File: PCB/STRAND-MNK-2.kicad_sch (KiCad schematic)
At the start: 4 parts

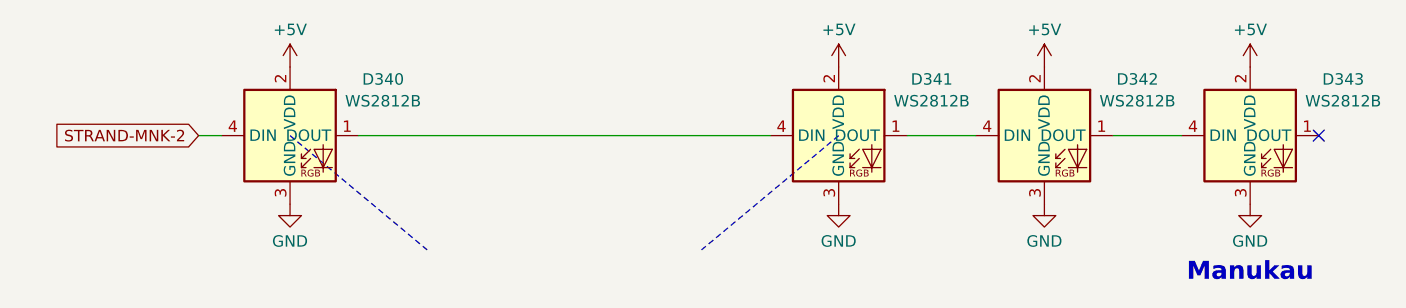
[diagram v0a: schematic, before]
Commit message: Final tweaks for V1.0.0
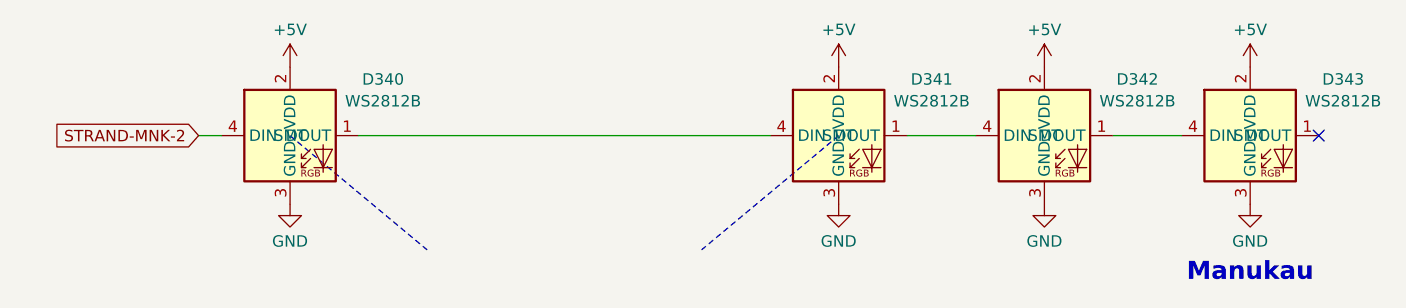
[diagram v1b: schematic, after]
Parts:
- D340, D341, D342, D343: Manufacturer (none) -> XINGLIGHT; Part (none) -> XL-1615RGBC-WS2812B; Process (none) -> SMT
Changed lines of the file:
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@@
+			)
+		)
+		(property "Part" "XL-1615RGBC-WS2812B"
+			(at 124.46 27.94 0)
+			(effects
+				(font
+					(size 1.27 1.27)
+				)
+				(hide yes)
+			)
+		)
+		(property "Manufacturer" "XINGLIGHT"
+			(at 124.46 27.94 0)
+			(effects
+				(font
+					(size 1.27 1.27)
+				)
+				(hide yes)
+			)
+		)
+		(property "PartID" ""
+			(at 124.46 27.94 0)
+			(effects
+				(font
+					(size 1.27 1.27)
+				)
+			)
+		)
+		(property "Process" "SMT"
+			(at 124.46 27.94 0)
+			(effects
+				(font
+					(size 1.27 1.27)
+				)
 			)
 		)
@@
 			)
 		)
+		(property "Part" "XL-1615RGBC-WS2812B"
+			(at 147.32 27.94 0)
+			(effects
+				(font
+					(size 1.27 1.27)
+				)
+				(hide yes)
+			)
+		)
+		(property "Manufacturer" "XINGLIGHT"
+			(at 147.32 27.94 0)
+			(effects
+				(font
+					(size 1.27 1.27)
+				)
+				(hide yes)
+			)
+		)
+		(property "PartID" ""
+			(at 147.32 27.94 0)
+			(effects
+				(font
+					(size 1.27 1.27)
+				)
+			)
+		)
+		(property "Process" "SMT"
+			(at 147.32 27.94 0)
+			(effects
+				(font
+					(size 1.27 1.27)
+				)
+			)
+		)
 		(pin "2"
 		)
@@
 			)
 		)
+		(property "Part" "XL-1615RGBC-WS2812B"
+			(at 101.6 27.94 0)
+			(effects
+				(font
+					(size 1.27 1.27)
+				)
+				(hide yes)
+			)
+		)
+		(property "Manufacturer" "XINGLIGHT"
+			(at 101.6 27.94 0)
+			(effects
+				(font
+					(size 1.27 1.27)
+				)
+				(hide yes)
+			)
+		)
+		(property "PartID" ""
+			(at 101.6 27.94 0)
+			(effects
+				(font
+					(size 1.27 1.27)
+				)
+			)
+		)
+		(property "Process" "SMT"
+			(at 101.6 27.94 0)
+			(effects
+				(font
+					(size 1.27 1.27)
+				)
+			)
+		)
 		(pin "2"
 		)
@@
 			)
 		)
+		(property "Part" "XL-1615RGBC-WS2812B"
+			(at 40.64 27.94 0)
+			(effects
+				(font
+					(size 1.27 1.27)
+				)
+				(hide yes)
+			)
+		)
+		(property "Manufacturer" "XINGLIGHT"
+			(at 40.64 27.94 0)
+			(effects
+				(font
+					(size 1.27 1.27)
+				)
+				(hide yes)
+			)
+		)
+		(property "PartID" ""
+			(at 40.64 27.94 0)
+			(effects
+				(font
+					(size 1.27 1.27)
+				)
+			)
+		)
+		(property "Process" "SMT"
+			(at 40.64 27.94 0)
+			(effects
+				(font
+					(size 1.27 1.27)
+				)
+			)
+		)
